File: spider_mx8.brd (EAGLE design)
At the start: 20 x 49.5 mm, 7 parts, among them IC1 AVR-MEGA8-PPTH, J1 AVR_SPI_PRG_6NS

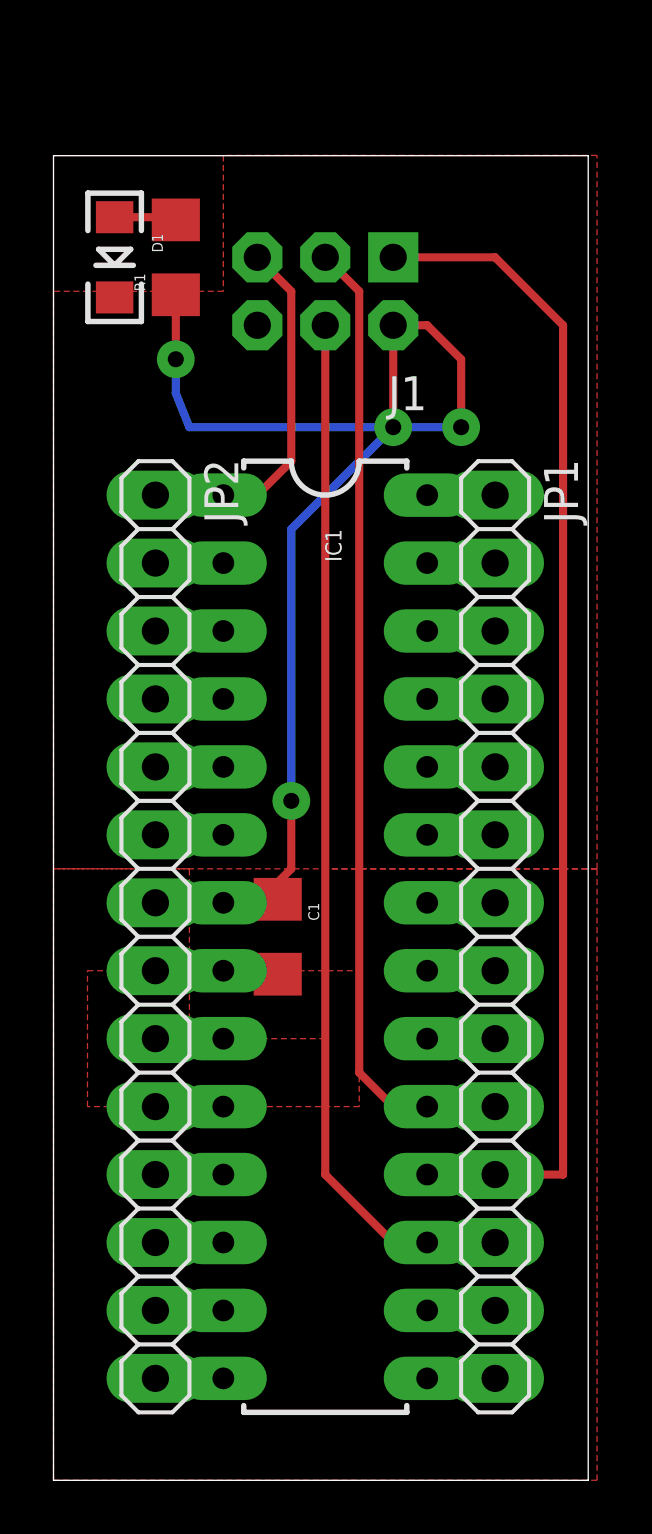
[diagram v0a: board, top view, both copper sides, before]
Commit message: printed this version out.  works.  sexy.
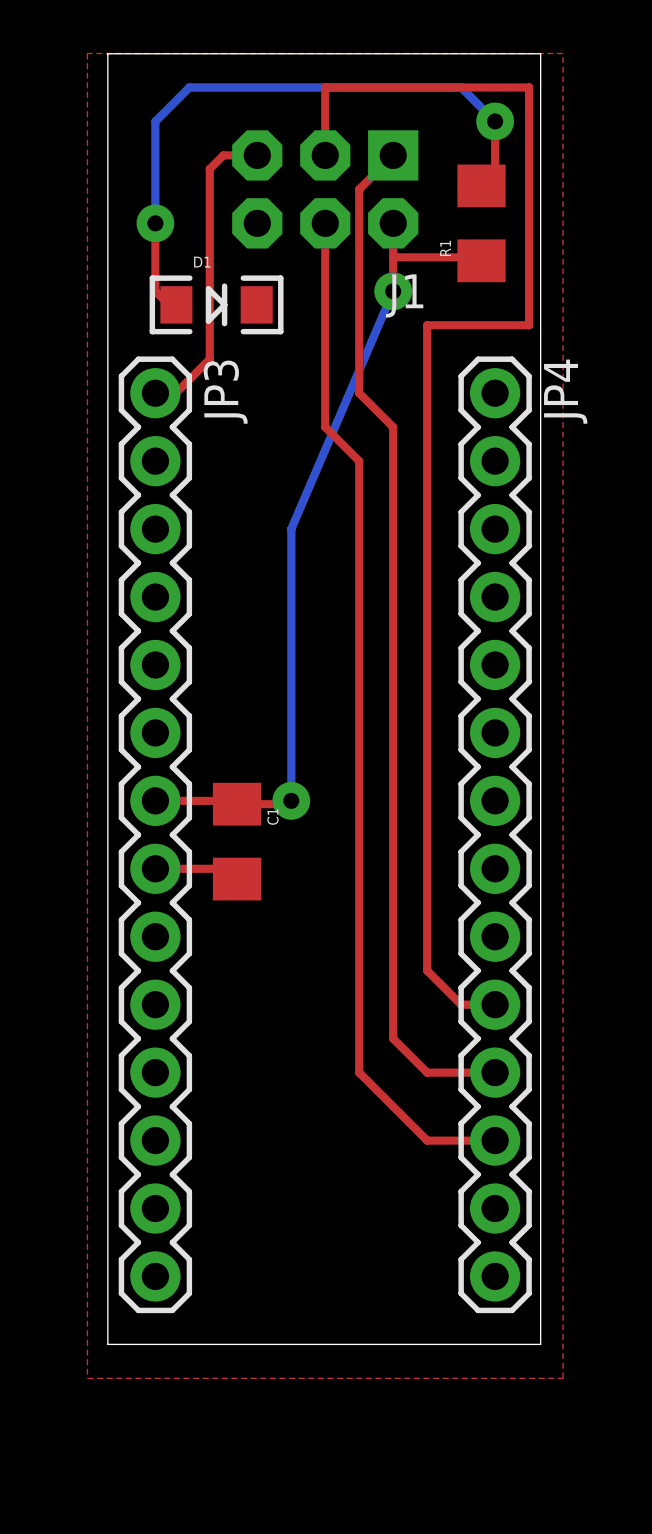
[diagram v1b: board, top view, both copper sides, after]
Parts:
- removed IC1: AVR-MEGA8-PPTH, SparkFun-DigitalIC:DIL28-3
- removed JP1, JP2: (no value), pinhead:1X14
- added JP3, JP4: M14, SparkFun-Connectors:1X14
- moved R1 11.5 mm to (49.0, 63.5)
- moved D1 4.20 mm to (39.1, 60.5), turned to 0 degrees
- moved C1 3.87 mm to (39.9, 40.4)
- moved J1 3.81 mm to (43.2, 64.8)
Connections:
- net GND: now also JP3.8; no longer IC1.8, JP2.8
- net MISO: now also JP4.11; no longer IC1.18, JP1.11
- net MOSI: now also JP4.12; no longer IC1.17, JP1.12
- net RESET: now also JP3.1; no longer IC1.1, JP2.1
- net SCK: now also JP4.10; no longer IC1.19, JP1.10
- net VCC: now also JP3.7; no longer IC1.7, JP2.7
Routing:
- net N$14: track 2.33 -> 23.7 mm, vias 0 -> 2
- net VCC: track 48.7 -> 31.0 mm, vias 4 -> 2
- net SCK: track 36.6 -> 50.1 mm
- net MISO: track 46.8 -> 38.4 mm
- net RESET: track 13.8 -> 11.7 mm
- net GND: track 4.63 -> 3.21 mm
- net MOSI: track 39.2 -> 38.4 mm
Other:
- board size 20 x 49.5 mm -> 16.2 x 48.2 mm
